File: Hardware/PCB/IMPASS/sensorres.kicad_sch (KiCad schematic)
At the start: 40 parts, among them J13 SENSORES, U12 MCP3008, U13 LM75B, U2 ACS712xLCTR-30A, U3 ACS712xLCTR-30A, U4 ACS712xLCTR-30A, U5 ACS712xLCTR-30A, U6 ACS712xLCTR-30A, U7 ACS712xLCTR-30A, U8 LM75B, U9 AS5047D

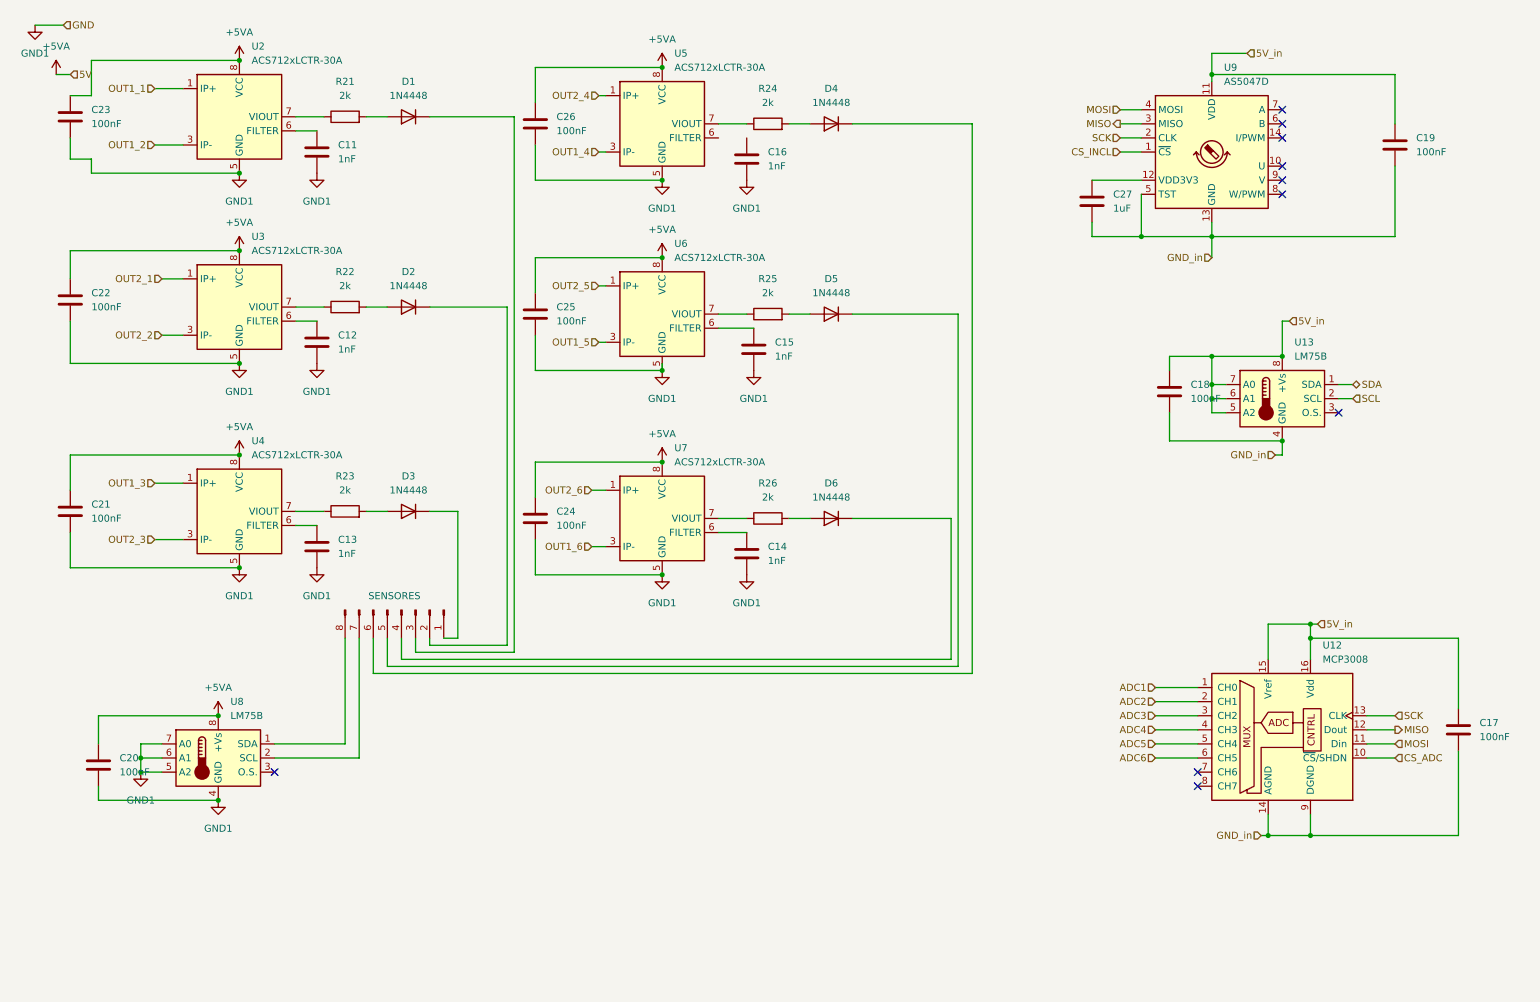
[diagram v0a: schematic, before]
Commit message: Update v1
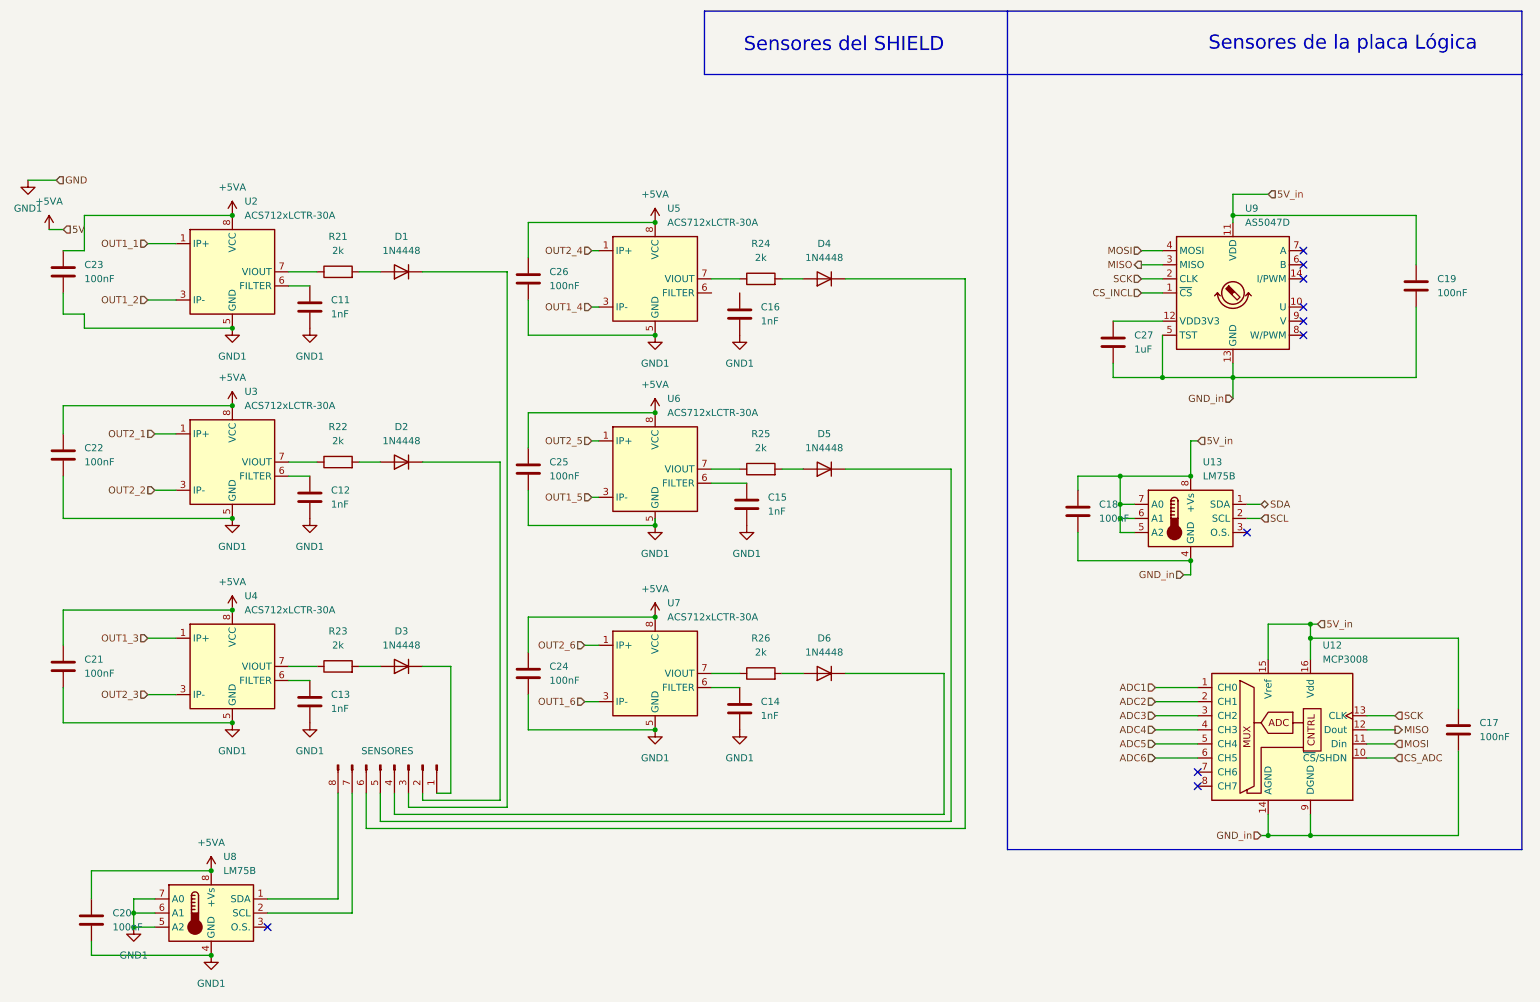
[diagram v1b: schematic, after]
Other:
- note added: "Sensores de la placa Lógica"
- note added: "Sensores del SHIELD"
- company: (none) -> Luis Miguel Carmona Cortés
- title: (none) -> IMPASS 
- moved on the sheet: C11, C12, C13, C14, C15, C16, C18, C19, C20, C21, C22, C23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
